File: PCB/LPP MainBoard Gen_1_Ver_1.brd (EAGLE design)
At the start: 50 x 115 mm, 48 parts, among them IC1 FE1.1S, U1 MAX15070, U3 BTN7933B, U4 MAX15070, U5 BTN7933B, U7 Pill STM32G431, U8 Blue Pill STM32F103

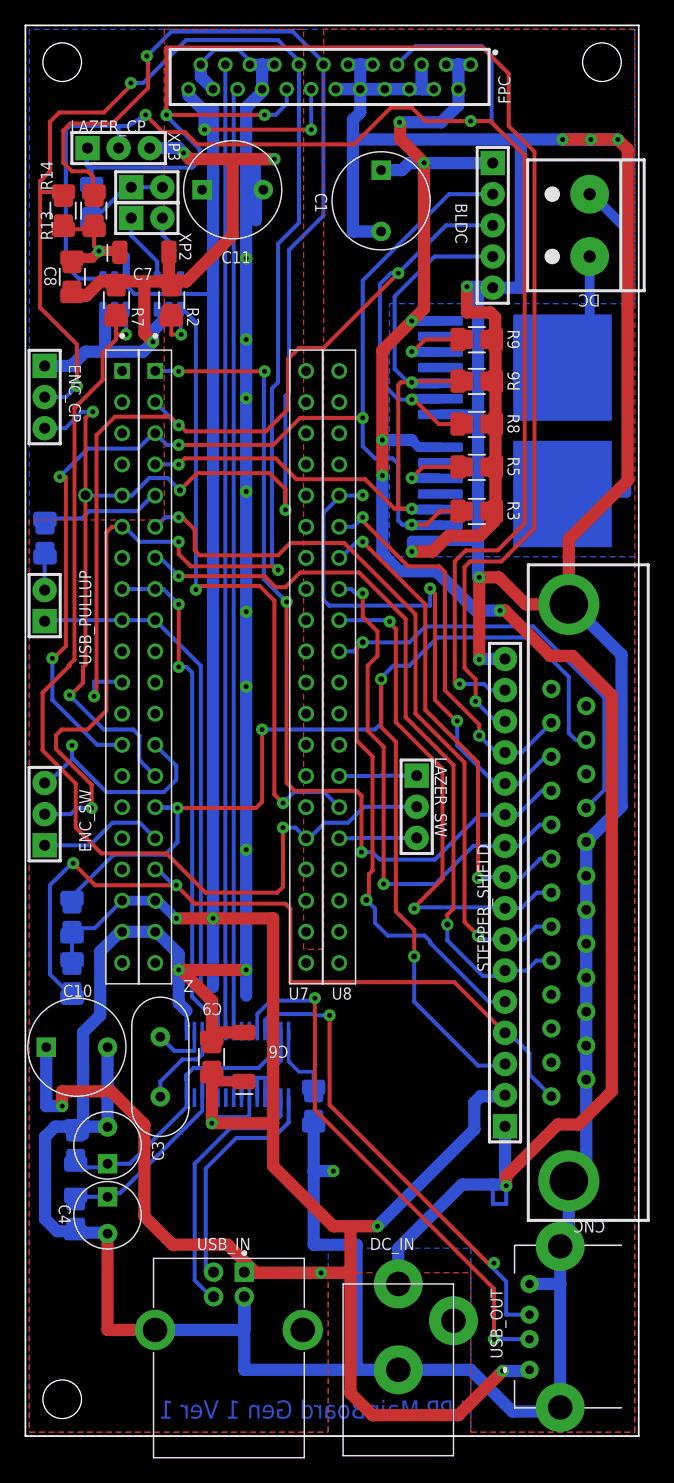
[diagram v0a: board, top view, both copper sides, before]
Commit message: modified:   PCB/LPP MainBoard Gen_1_Ver_1.brd 	deleted:    "PCB/LPP_MainBoard_Gen_1_Ver_1 \342\200\224 \320\272\320\276\320\277\320\270\321\217.dch" 	deleted:    "PCB/LPP_MainBoard_Gen_1_Ver_1 \342\200\224 \320\272\320\276\320\277\320\270\321\217.dip" 	modified:   PCB/LPP_MainBoard_Gen_1_Ver_1.dip
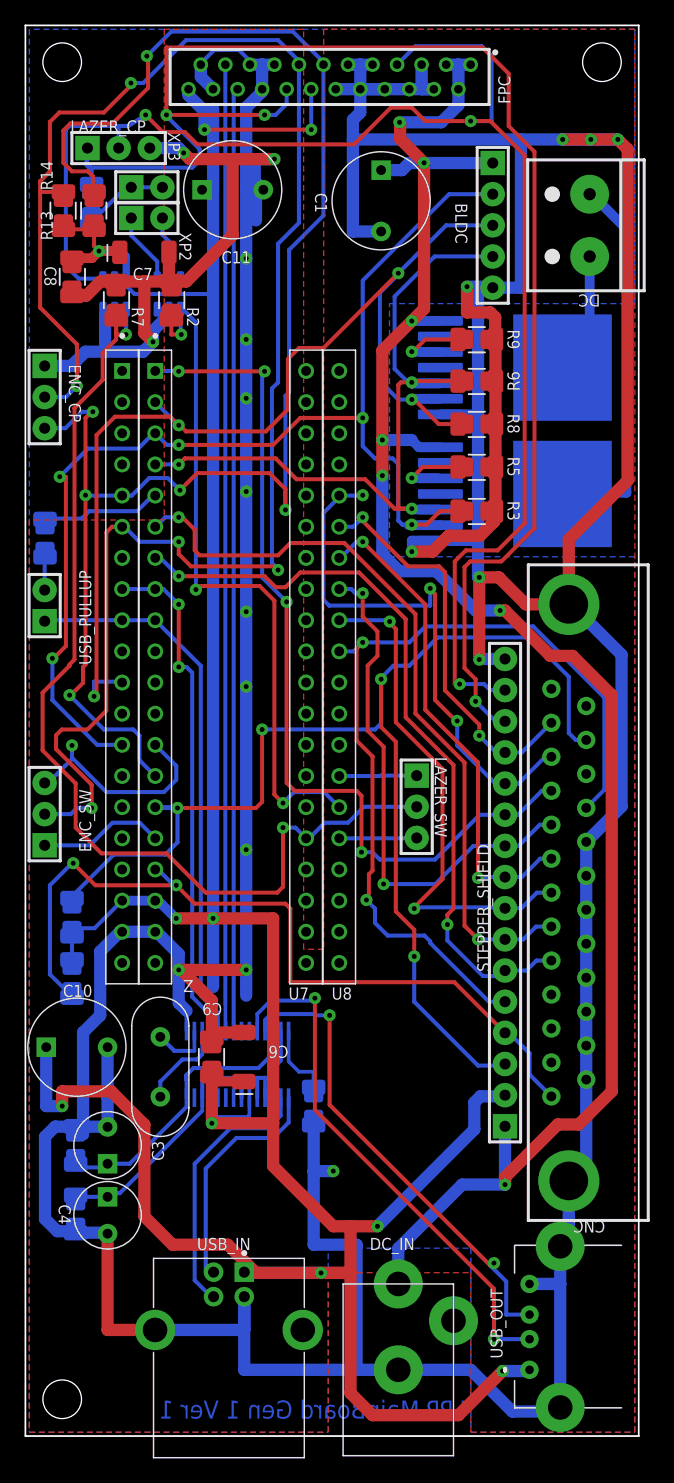
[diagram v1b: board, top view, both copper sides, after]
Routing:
- net Сеть_16: track 155.6 -> 151.2 mm
